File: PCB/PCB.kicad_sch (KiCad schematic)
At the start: 44 parts, among them J1 440054-2, J2 USB_C_Receptacle_PowerOnly_6P, Q1 IRLML6402, Q2 IRLML6402, Q3 2N3904, Q4 2N3904, SW1 SW_SPDT_312, U1 DRV8833PWPR, U2 DRV8833PWPR, U3 INA219AxD, U4 CH224K, U5 L6924D, U6 SN74HC4066PWR

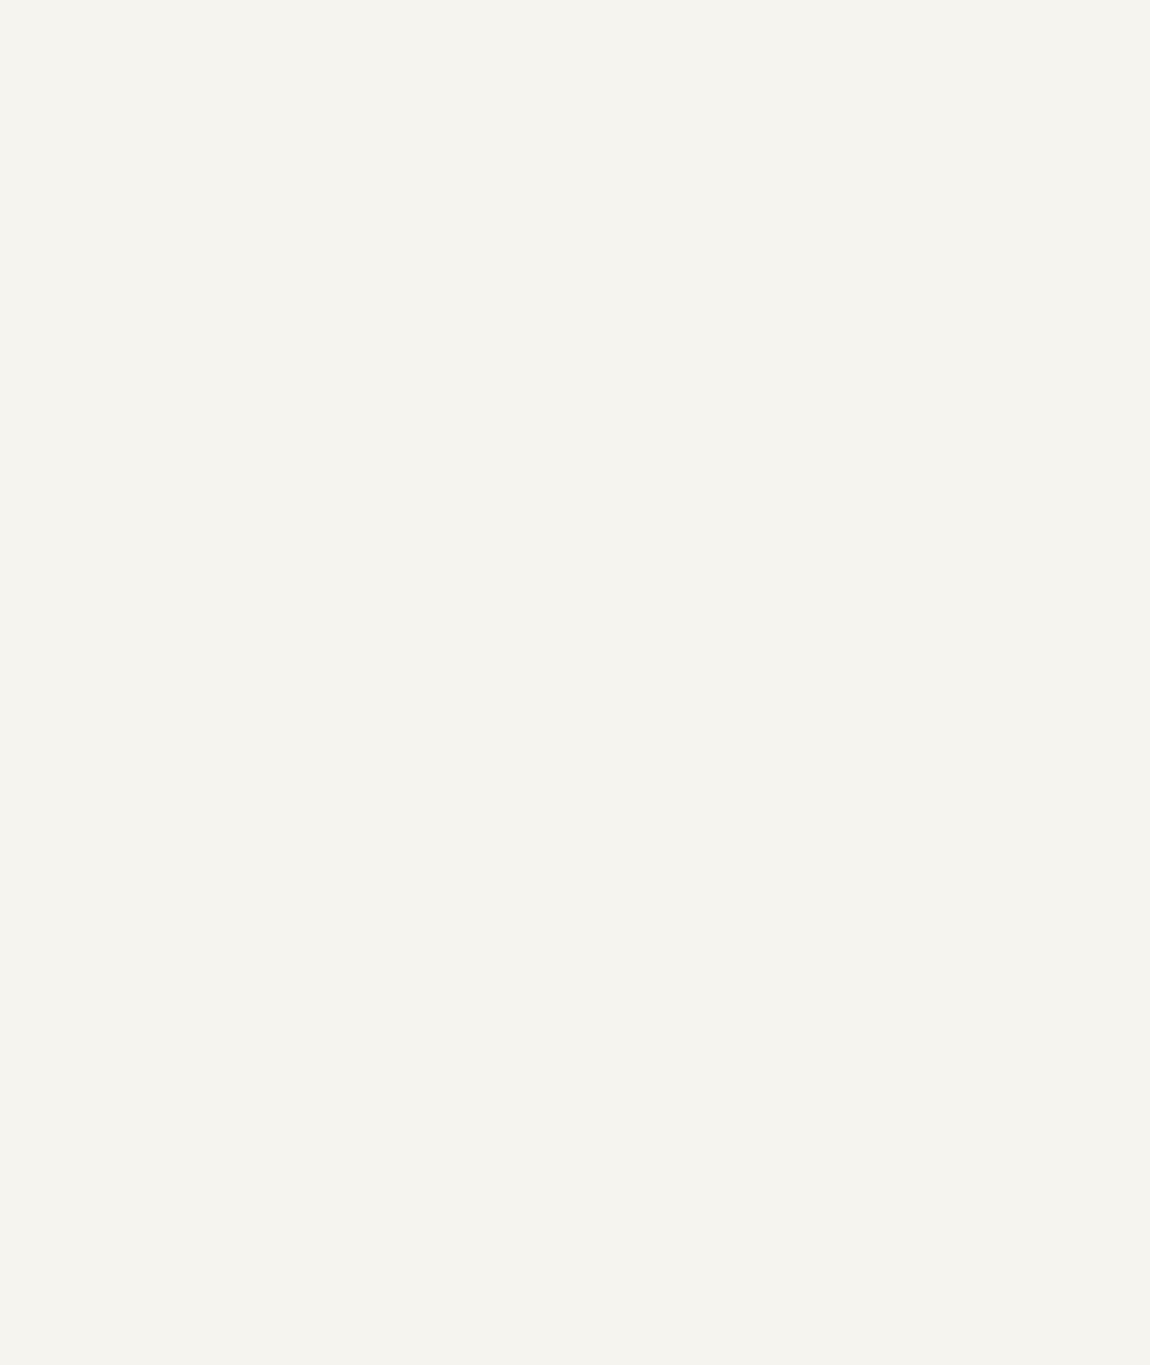
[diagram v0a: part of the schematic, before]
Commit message: 3V3 and 5V
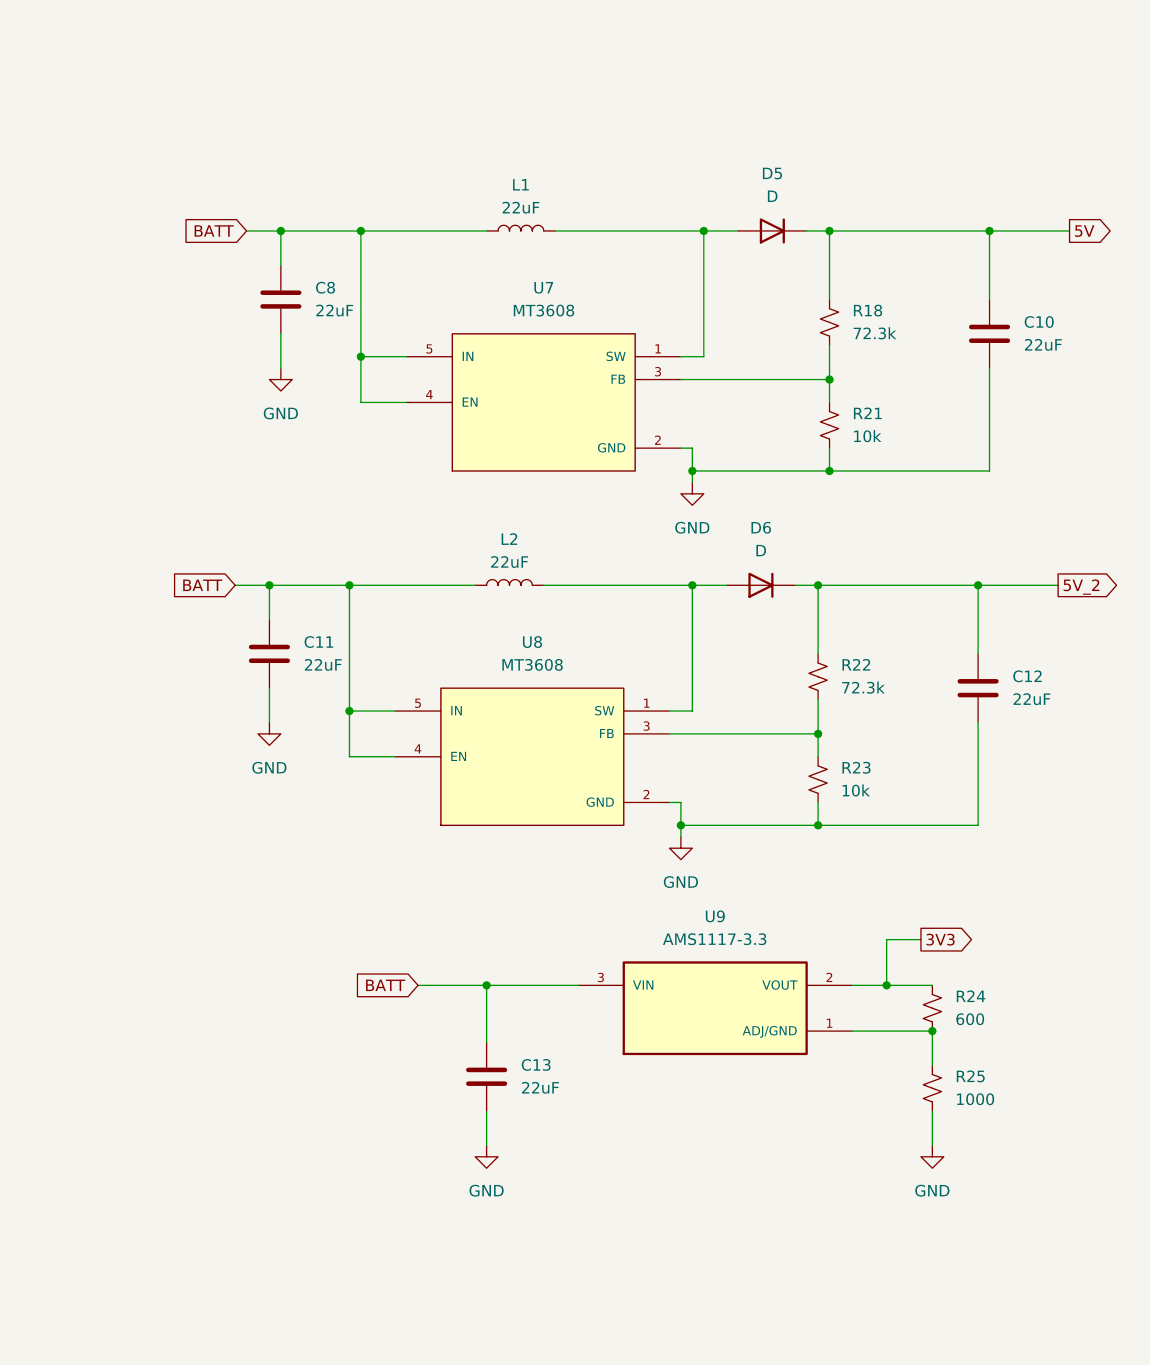
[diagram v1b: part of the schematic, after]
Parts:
- added C10, C11, C12, C13, C8: 22uF, symbol Device:C
- added D5, D6: D, symbol Device:D
- added L1, L2: 22uF, symbol Device:L
- added R18, R22: 72.3k, symbol Device:R_Small_US
- added R21, R23: 10k, symbol Device:R_Small_US
- added R24: 600, symbol Device:R_Small_US
- added R25: 1000, symbol Device:R_Small_US
- added U7, U8: MT3608, MT3608:SOT95P280X145-6N, symbol MT3608:MT3608
- added U9: AMS1117-3.3, AMS1117-3.3:SOT229P700X180-4N, symbol AMS1117-3.3:AMS1117-3.3
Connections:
- net 3V3: now also R24.1, U9.2 (VOUT)
- net 5V: now also C10.1, D5.1 (K), R18.1
- net BATT: now also C11.1, C13.1, C8.1, L1.1, L2.1, U7.4 (EN), U7.5 (IN), U8.4 (EN), U8.5 (IN), U9.3 (VIN)
- net GND: now also C10.2, C11.2, C12.2, C13.2, C8.2, R21.2, R23.2, R25.2, U7.2 (GND), U8.2 (GND)
- new net: R24.2, R25.1, U9.1 (ADJ/GND)
- new net: D6.2 (A), L2.2, U8.1 (SW)
- new net: R22.2, R23.1, U8.3 (FB)
- new net: D5.2 (A), L1.2, U7.1 (SW)
- new net: R18.2, R21.1, U7.3 (FB)
- new net 5V_2: C12.1, D6.1 (K), R22.1
